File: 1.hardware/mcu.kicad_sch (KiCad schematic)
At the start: 35 parts, among them IC3 STWD100NXWY3F, J2 Conn_01x02, J3 Debug, SW2 SW_DPDT_x2, SW3 Reset_Btn, U1 STM32H743BITx, X1 SMD3225-4

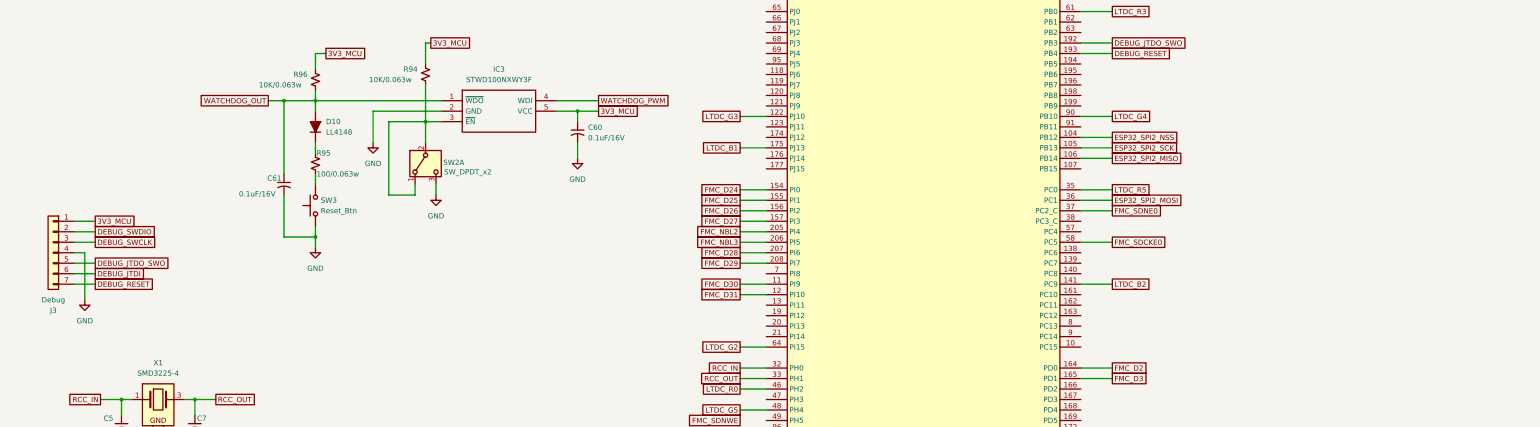
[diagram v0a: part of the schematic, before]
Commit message: 중간 저장
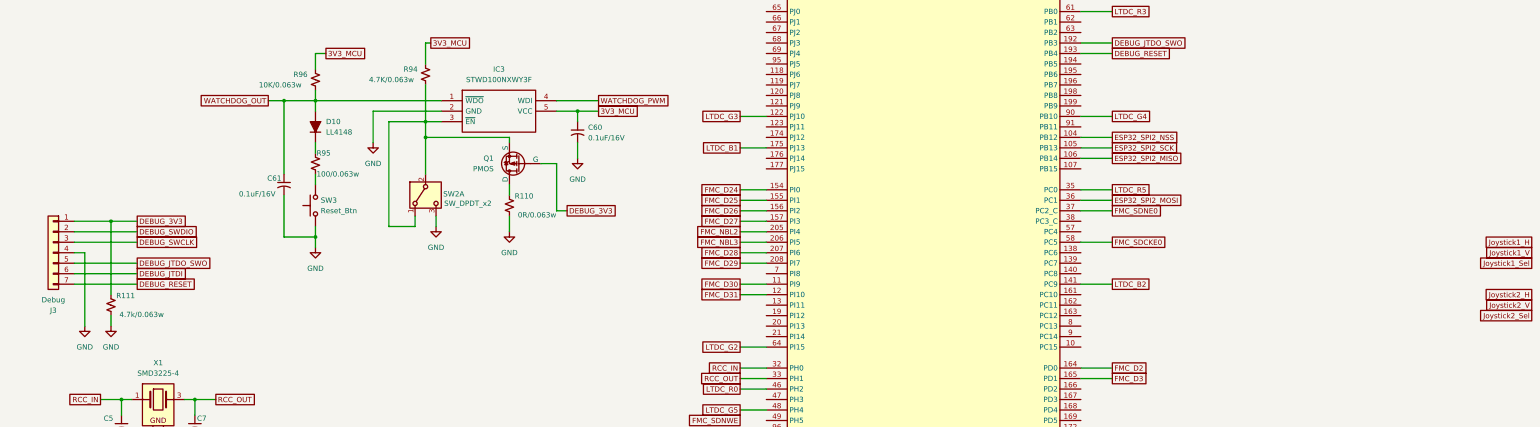
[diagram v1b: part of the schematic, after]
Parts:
- added Q1: PMOS, symbol Simulation_SPICE:PMOS
- added R110: 0R/0.063w, Resistor_SMD:R_0402_1005Metric, symbol Device:R_Small_US
- added R111: 4.7k/0.063w, Resistor_SMD:R_0402_1005Metric, symbol Device:R_Small_US
- IC3: footprint SOT95P280X145-5N -> SamacSys_Parts:SOT95P280X145-5N
- R94: value 10K/0.063w -> 4.7K/0.063w; footprint (none) -> Resistor_SMD:R_0402_1005Metric
- R95, R96: footprint (none) -> Resistor_SMD:R_0402_1005Metric
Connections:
- net 3V3_MCU: no longer J3.1 (Pin_1)
- net GND: now also R110.2, R111.2
- net at IC3.3 (~{EN}), R94.2, SW2.1 (A)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: now also Q1.3 (S)
- new net: Q1.1 (D), R110.1
- new net DEBUG_3V3: J3.1 (Pin_1), Q1.2 (G), R111.1
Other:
- moved on the sheet: SW2A

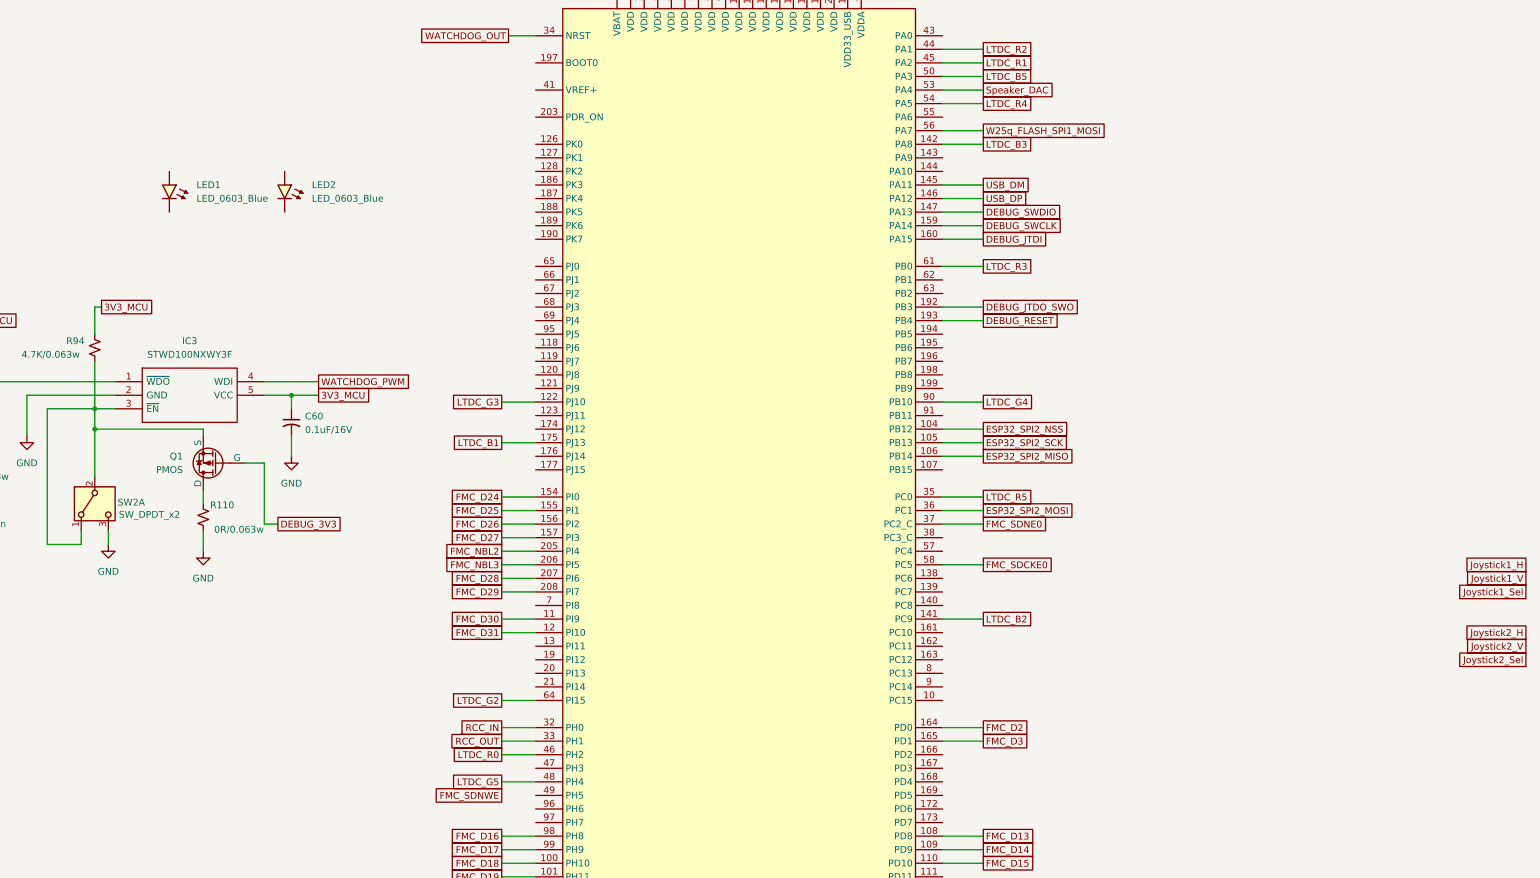
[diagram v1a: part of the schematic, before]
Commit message: 중간 저장
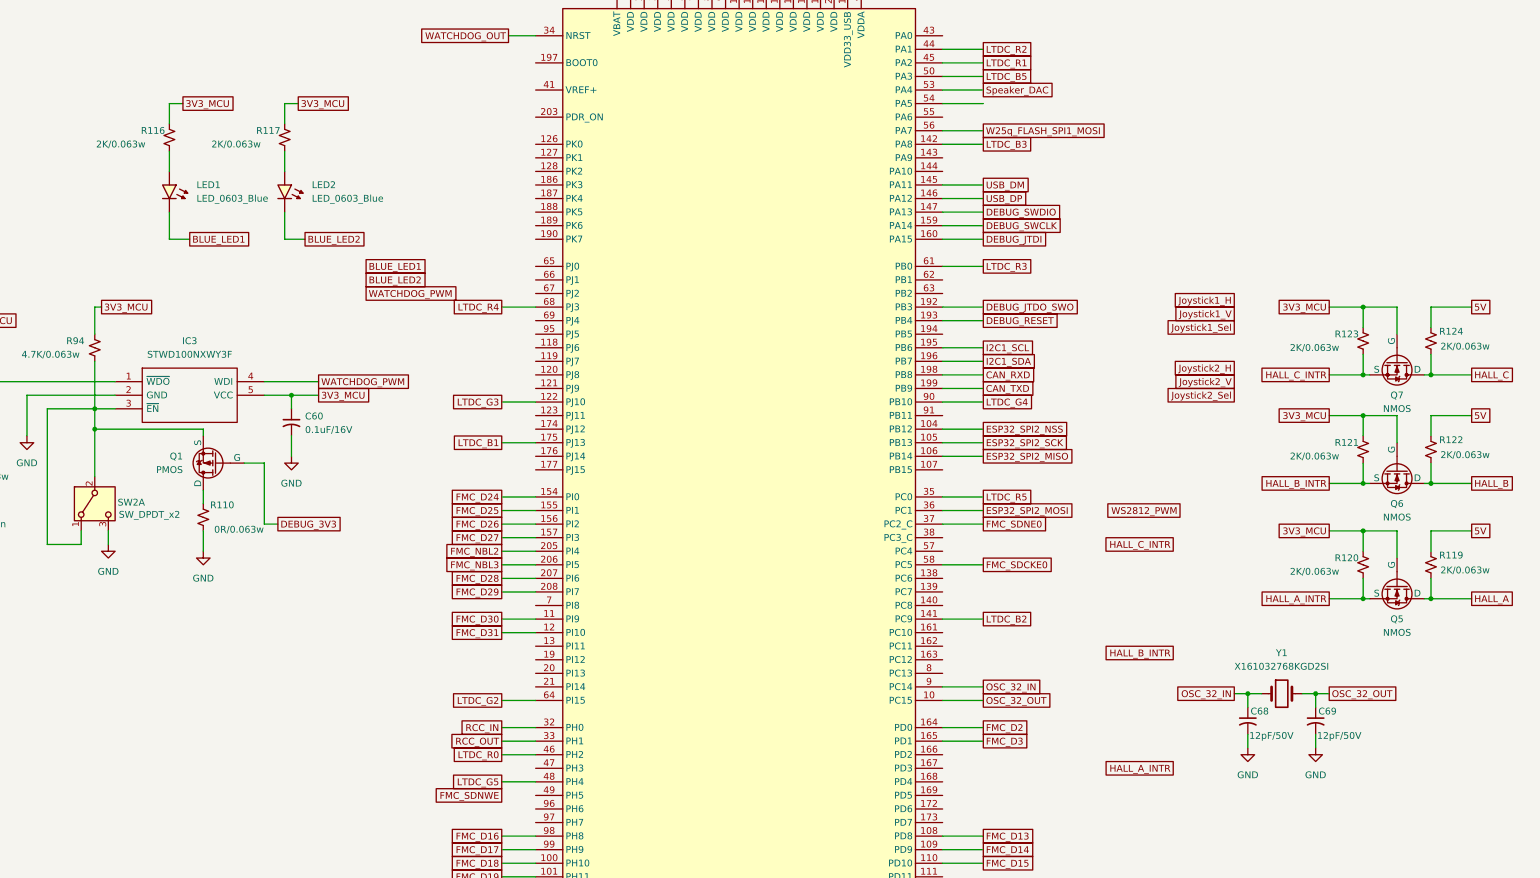
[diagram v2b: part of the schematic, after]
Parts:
- added C68, C69: 12pF/50V, symbol Device:C_Small_US
- added Q5, Q6, Q7: NMOS, symbol Simulation_SPICE:NMOS
- added R116, R117, R119, R120, R121, R122, R123, R124: 2K/0.063w, Resistor_SMD:R_0402_1005Metric, symbol Device:R_Small_US
- added Y1: X161032768KGD2SI, symbol Device:Crystal
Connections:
- net 3V3_MCU: now also Q5.2 (G), Q6.2 (G), Q7.2 (G), R116.1, R117.1, R120.1, R121.1, R123.1
- net GND: now also C68.2, C69.2
- net LTDC_R4: now also U1.68 (PJ3); no longer U1.54 (PA5)
- net BLUE_LED2: now reaches LED2.1 (K)
- net at LED2.2 (A): now also R117.2
- net BLUE_LED1: now reaches LED1.1 (K)
- net at LED1.2 (A): now also R116.2
- net OSC_32_OUT: now reaches U1.10 (PC15)
- net OSC_32_OUT: now also C69.1, Y1.2
- net I2C1_SCL: now reaches U1.195 (PB6)
- net I2C1_SDA: now reaches U1.196 (PB7)
- net CAN_RXD: now reaches U1.198 (PB8)
- net CAN_TXD: now reaches U1.199 (PB9)
- net OSC_32_IN: now reaches U1.9 (PC14)
- net OSC_32_IN: now also C68.1, Y1.1
- new net 5V: R119.1, R122.1, R124.1
- new net HALL_A: Q5.1 (D), R119.2
- new net HALL_A_INTR: Q5.3 (S), R120.2
- new net HALL_B: Q6.1 (D), R122.2
- new net HALL_B_INTR: Q6.3 (S), R121.2
- new net HALL_C: Q7.1 (D), R124.2
- new net HALL_C_INTR: Q7.3 (S), R123.2

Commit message: 중간 수정
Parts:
- C68, C69: footprint (none) -> Capacitor_SMD:C_0402_1005Metric
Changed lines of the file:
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@@
 			)
 		)
-		(property "Footprint" ""
+		(property "Footprint" "Capacitor_SMD:C_0402_1005Metric"
 			(at 378.46 209.55 0)
 			(effects
@@
 			)
 		)
-		(property "Footprint" ""
+		(property "Footprint" "Capacitor_SMD:C_0402_1005Metric"
 			(at 391.16 209.55 0)
 			(effects
